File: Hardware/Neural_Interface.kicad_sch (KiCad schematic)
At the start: 8 parts, among them SW1 RESET, SW2 BOOT

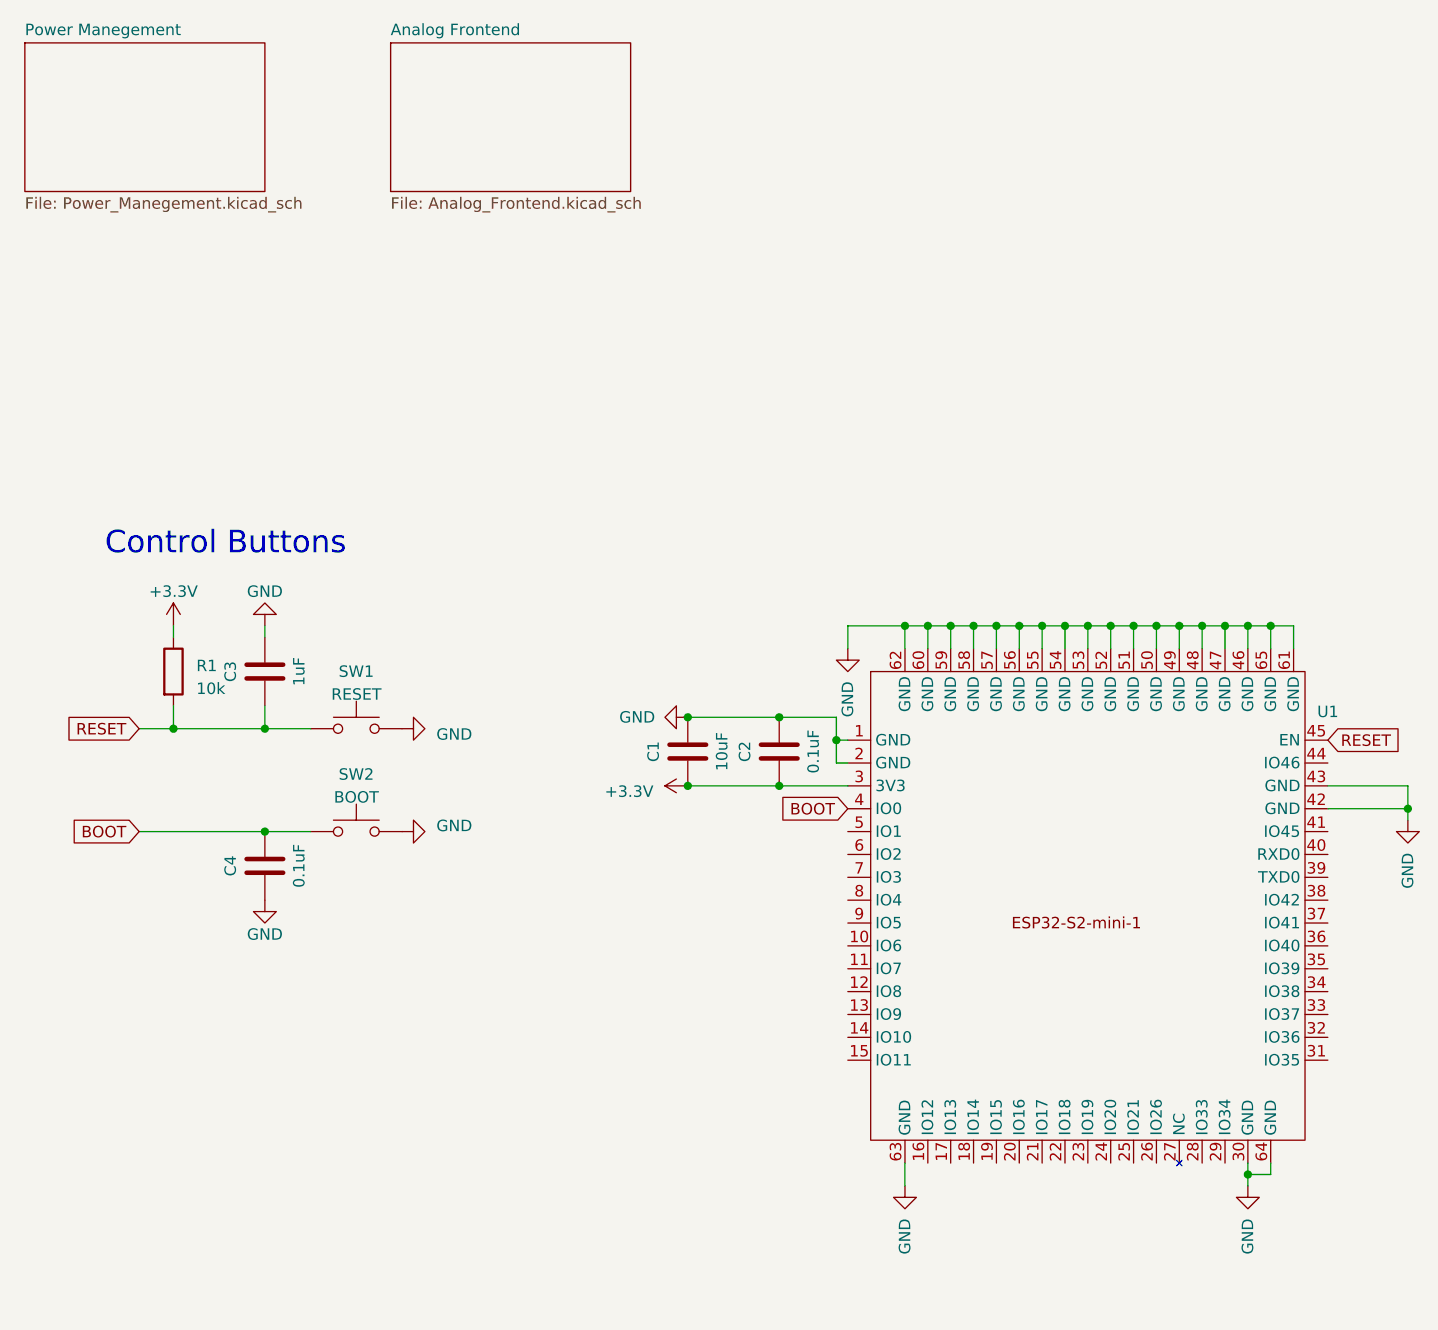
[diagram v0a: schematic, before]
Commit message: Power Management Complete
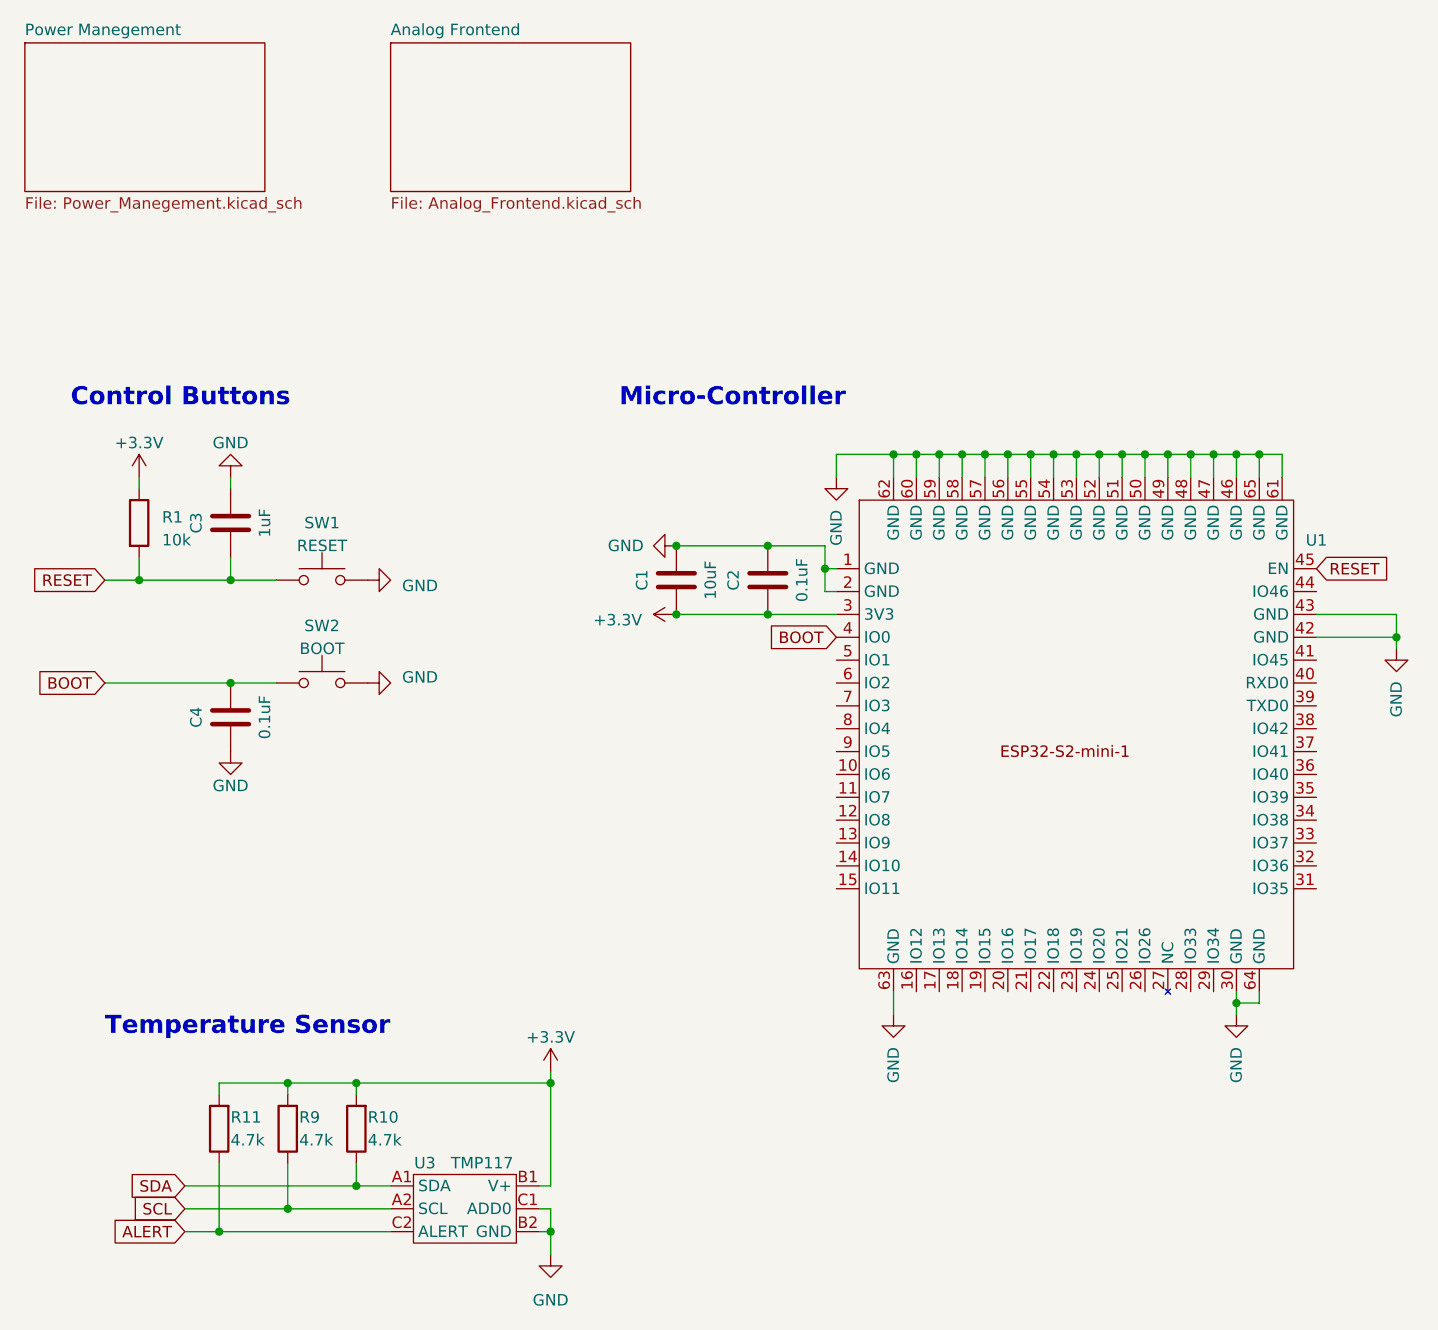
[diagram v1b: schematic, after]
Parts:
- added R10, R11, R9: 4.7k, Resistor_SMD:R_0402_1005Metric, symbol Device:R
- added U3: TMP117, Package_BGA:Texas_DSBGA-6_0.95x1.488mm_Layout2x3_P0.4mm, symbol Motor_Driver:TMP117
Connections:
- net +3.3V: now also R10.2, R11.2, R9.2, U3.B1 (V+)
- net GND: now also U3.B2 (GND), U3.C1 (ADD0)
- new net ALERT: R11.1, U3.C2 (ALERT)
- new net SCL: R9.1, U3.A2 (SCL)
- new net SDA: R10.1, U3.A1 (SDA)
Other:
- note added: "Micro-Controller"
- note added: "Temperature Sensor"
- moved on the sheet: C1, C2, C3, C4, R1, SW1, SW2, U1
